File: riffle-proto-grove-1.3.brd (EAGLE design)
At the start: 48.9 x 17.8 mm, 20 parts, among them J9 A0

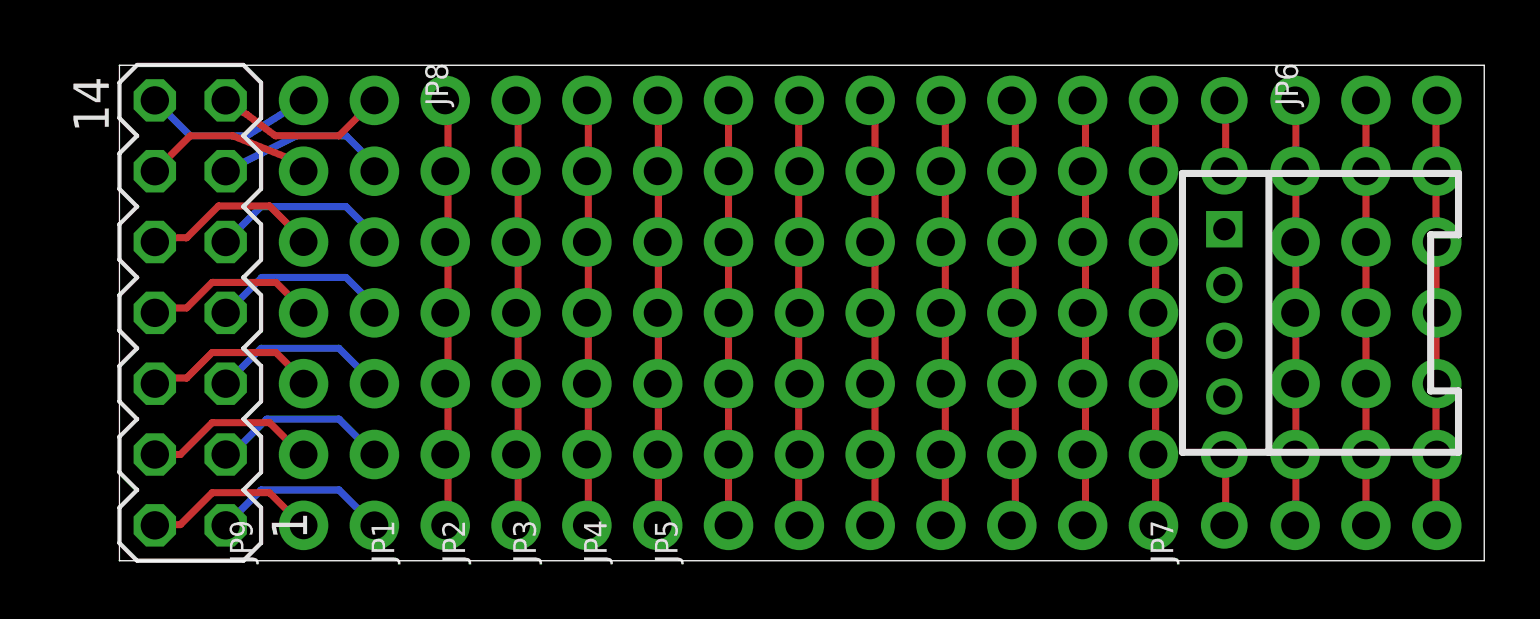
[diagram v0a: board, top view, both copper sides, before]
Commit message: update
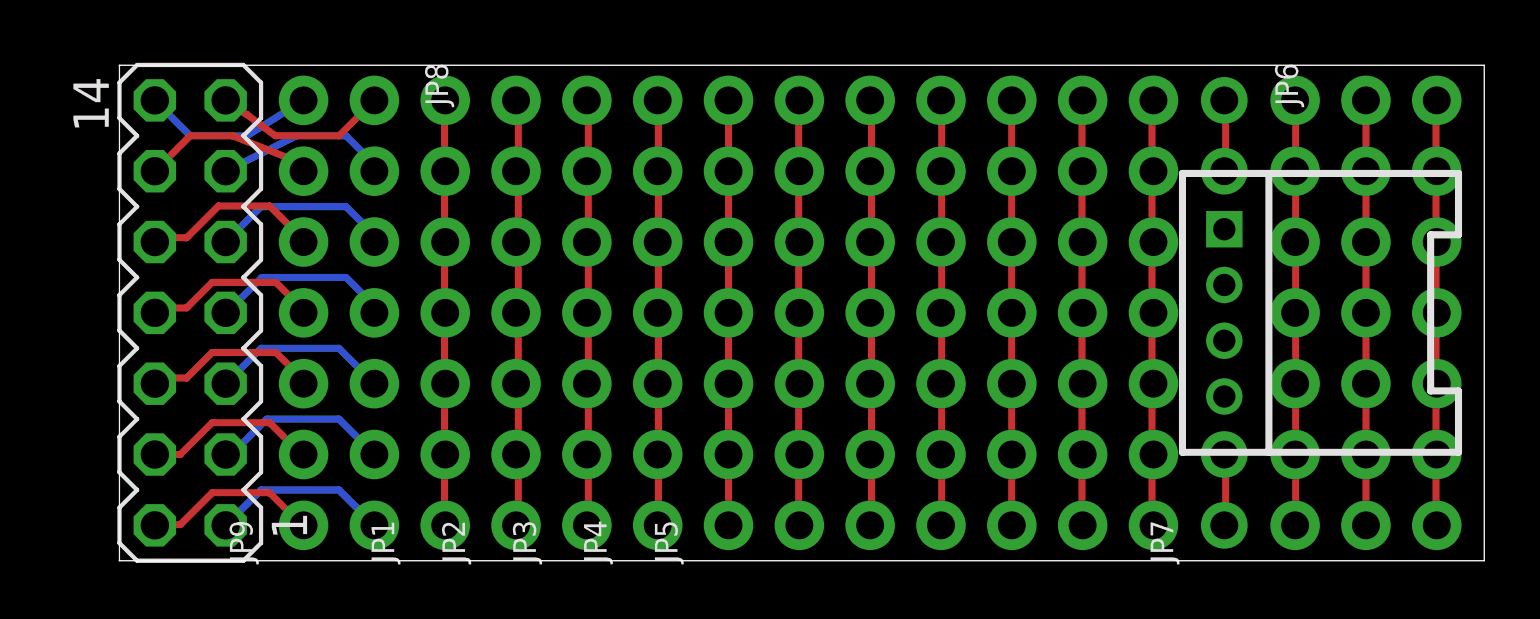
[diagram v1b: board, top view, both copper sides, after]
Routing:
- net N$9: track 16.5 -> 15.5 mm
- net N$12: track 16.2 -> 15.3 mm
- net N$13: track 16.0 -> 15.3 mm
